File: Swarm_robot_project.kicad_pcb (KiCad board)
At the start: 2 copper layers, 62.8 x 62.8 mm, 87 parts, among them J1 Motor_A, J2 Motor_B, J3 SW, J4 Lipo_2000mAh, J5 USB_C_Receptacle_USB2.0_16P, SW1 SW_Push, SW2 SW_Push, SW3 SW_SPDT, SW4 SW_Push, SW5 SW_POWER, U1 TPS63802DLAR, U2 MT3608, U3 BQ24075RGT, U4 DRV8833PWP, U5 STM32F103C8T6, U6 ESP32-C3-WROOM-02, U7 USBLC6-2SC6, Y1 16MHz

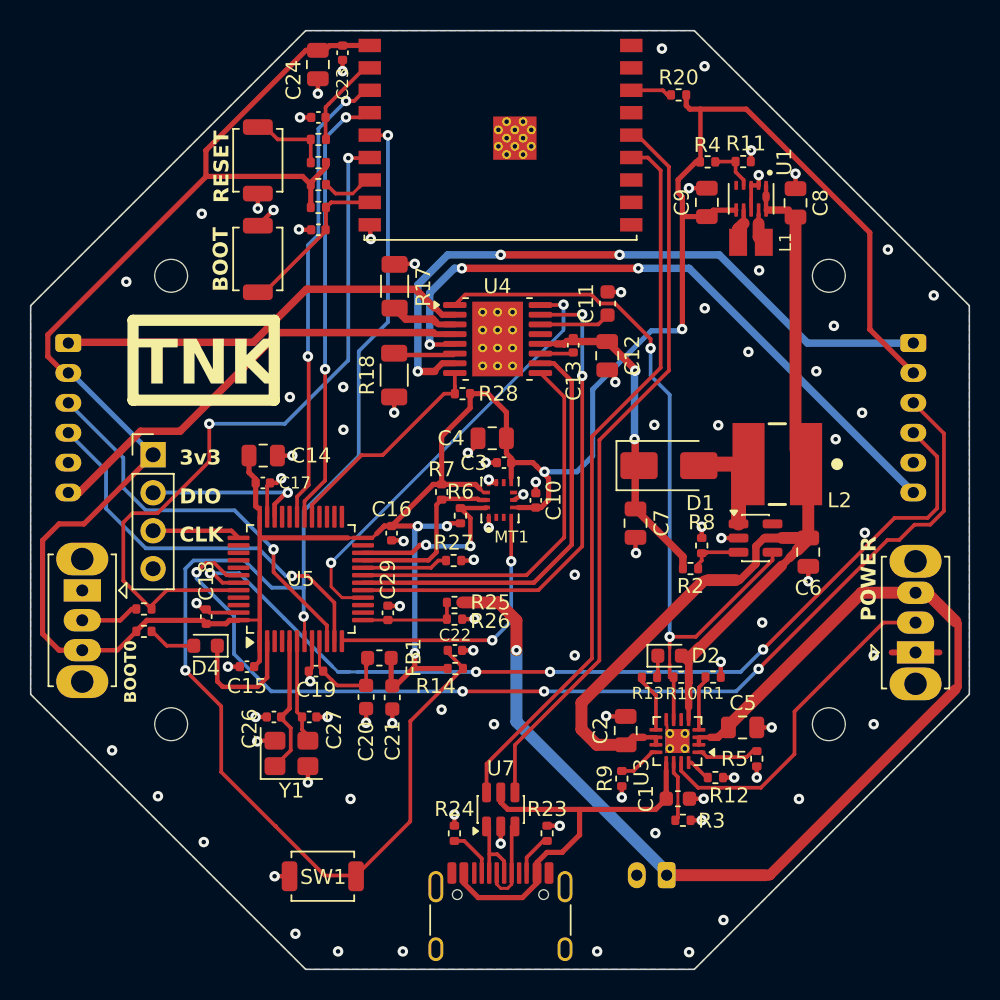
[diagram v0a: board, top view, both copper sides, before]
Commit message: UPDATE
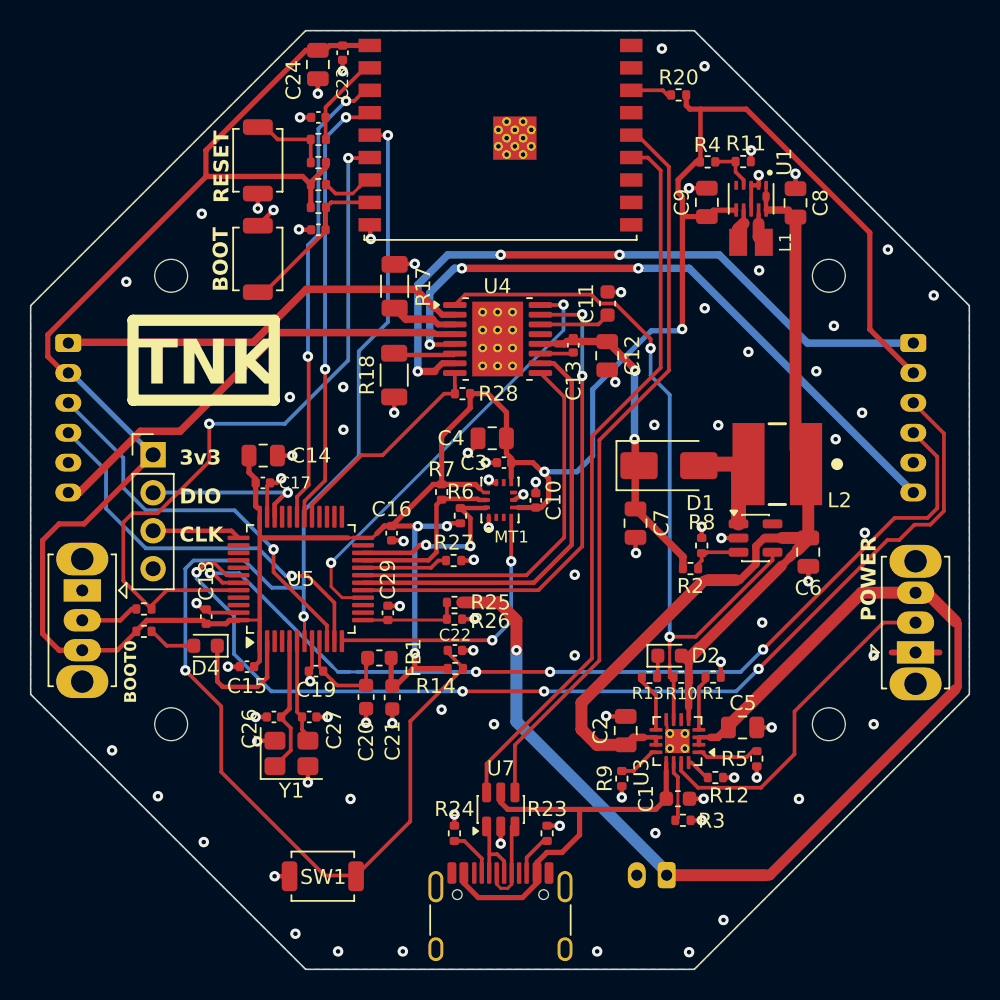
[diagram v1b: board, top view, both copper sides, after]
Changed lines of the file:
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@@
 			)
 		)
-		(property "LCSC" "C1525"
+		(property "LCSC" "C52923"
 			(at 0 0 0)
 			(layer "F.Fab")
@@
 	)
 	(segment
+		(start 175.45 41.47)
+		(end 175.45 40.85)
+		(width 0.2)
+		(layer "F.Cu")
+		(net "/VOUT")
+	)
+	(segment
 		(start 175.45 42.6125)
 		(end 175.45 42.5)
@@
 	)
 	(segment
-		(start 175.45 41.2125)
-		(end 175.45 40.85)
-		(width 0.3)
-		(layer "F.Cu")
-		(net "/VOUT")
-	)
-	(segment
 		(start 174.7702 64.992616)
 		(end 175.317516 64.4453)
@@
 	)
 	(segment
-		(start 175.45 41.47)
-		(end 175.45 41.2125)
-		(width 0.2)
-		(layer "F.Cu")
-		(net "/VOUT")
-	)
-	(segment
 		(start 154.6272 52.1052)
 		(end 154.5324 52.2)
@@
 	)
 	(segment
-		(start 153.15 49.8)
-		(end 151.3375 49.8)
-		(width 0.5)
+		(start 153.5052 50.1552)
+		(end 154.6272 50.1552)
+		(width 0.4)
 		(layer "F.Cu")
 		(net "Net-(U4-AISEN)")
 	)
 	(segment
-		(start 153.5052 50.1552)
-		(end 154.6272 50.1552)
-		(width 0.4)
+		(start 153.15 49.8)
+		(end 151.3375 49.8)
+		(width 0.5)
 		(layer "F.Cu")
 		(net "Net-(U4-AISEN)")
@@
 	)
 	(segment
-		(start 153.35 50)
-		(end 153.15 49.8)
-		(width 0.5)
+		(start 153.15 49.8)
+		(end 153.5052 50.1552)
+		(width 0.4)
 		(layer "F.Cu")
 		(net "Net-(U4-AISEN)")
@@
 	)
 	(segment
-		(start 136.25 57.3)
-		(end 133.6 57.3)
+		(start 133.6 57.3)
+		(end 136.25 57.3)
 		(width 0.5)
 		(layer "F.Cu")
@@
 	)
 	(segment
-		(start 133.6 57.3)
-		(end 129.5 61.4)
+		(start 129.5 61.4)
+		(end 133.6 57.3)
 		(width 0.5)
 		(layer "F.Cu")
@@
 	)
 	(segment
-		(start 142.85 50.7)
-		(end 136.25 57.3)
+		(start 136.25 57.3)
+		(end 142.85 50.7)
 		(width 0.5)
 		(layer "F.Cu")
@@
 	)
 	(segment
-		(start 129.5 61.4)
-		(end 128.77 61.4)
+		(start 154.6272 50.8052)
+		(end 153.315861 50.8052)
+		(width 0.4)
+		(layer "F.Cu")
+		(net "AOUT2")
+	)
+	(segment
+		(start 128.77 61.4)
+		(end 129.5 61.4)
 		(width 0.5)
 		(layer "F.Cu")
@@
 	)
 	(segment
-		(start 154.6272 50.8052)
-		(end 153.3052 50.8052)
-		(width 0.4)
+		(start 142.85 50.7)
+		(end 153.06005 50.7)
+		(width 0.5)
 		(layer "F.Cu")
 		(net "AOUT2")
 	)
 	(segment
-		(start 153.3052 50.8052)
-		(end 153.2 50.7)
+		(start 153.315861 50.8052)
+		(end 153.210661 50.7)
 		(width 0.4)
 		(layer "F.Cu")
@@
 	)
 	(segment
-		(start 153.2 50.7)
-		(end 142.85 50.7)
-		(width 0.5)
+		(start 153.210661 50.7)
+		(end 153.06005 50.7)
+		(width 0.4)
 		(layer "F.Cu")
 		(net "AOUT2")
@@
 		(width 0.25)
 		(layer "F.Cu")
-		(net "/NRST")
-	)
-	(segment
-		(start 142.625 83.725)
-		(end 142.65 83.7)
-		(width 0.25)
-		(layer "F.Cu")
